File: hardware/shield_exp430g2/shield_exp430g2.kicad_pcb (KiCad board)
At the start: 2 copper layers, 58.7 x 51.2 mm, 45 parts, among them J1 Digital, J10 Conn_01x02_Male, J11 Conn_01x02_Male, J12 Conn_01x02_Male, J13 Conn_01x02_Male, J14 Conn_01x04_Male, J15 Conn_01x02_Male, J16 Conn_01x02_Male, J17 Conn_01x02_Male, J18 Conn_01x02_Male, J19 Conn_01x02_Male, J2 Digital, J20 Conn_01x02_Male, J21 Conn_01x02_Male, J22 Conn_01x02_Male, J23 Conn_01x02_Male, J24 Conn_01x02_Male, J3 Conn_01x02_Male, J4 Conn_01x02_Male, J5 Conn_01x02_Male, J6 Conn_01x02_Male, J7 Conn_01x02_Male, J8 Conn_01x02_Male, J9 Conn_02x13_Odd_Even, U1 NCP1117-3.3_SOT223

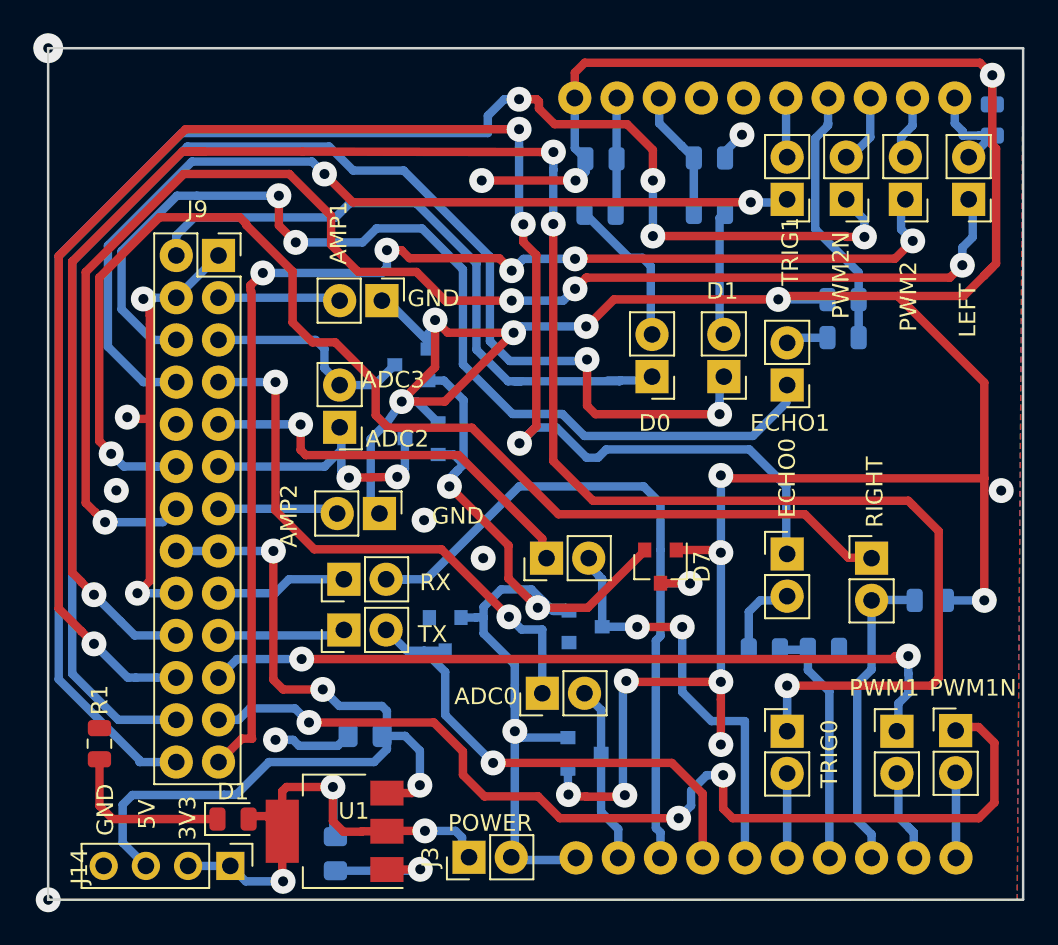
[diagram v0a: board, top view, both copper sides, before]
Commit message: Added diode
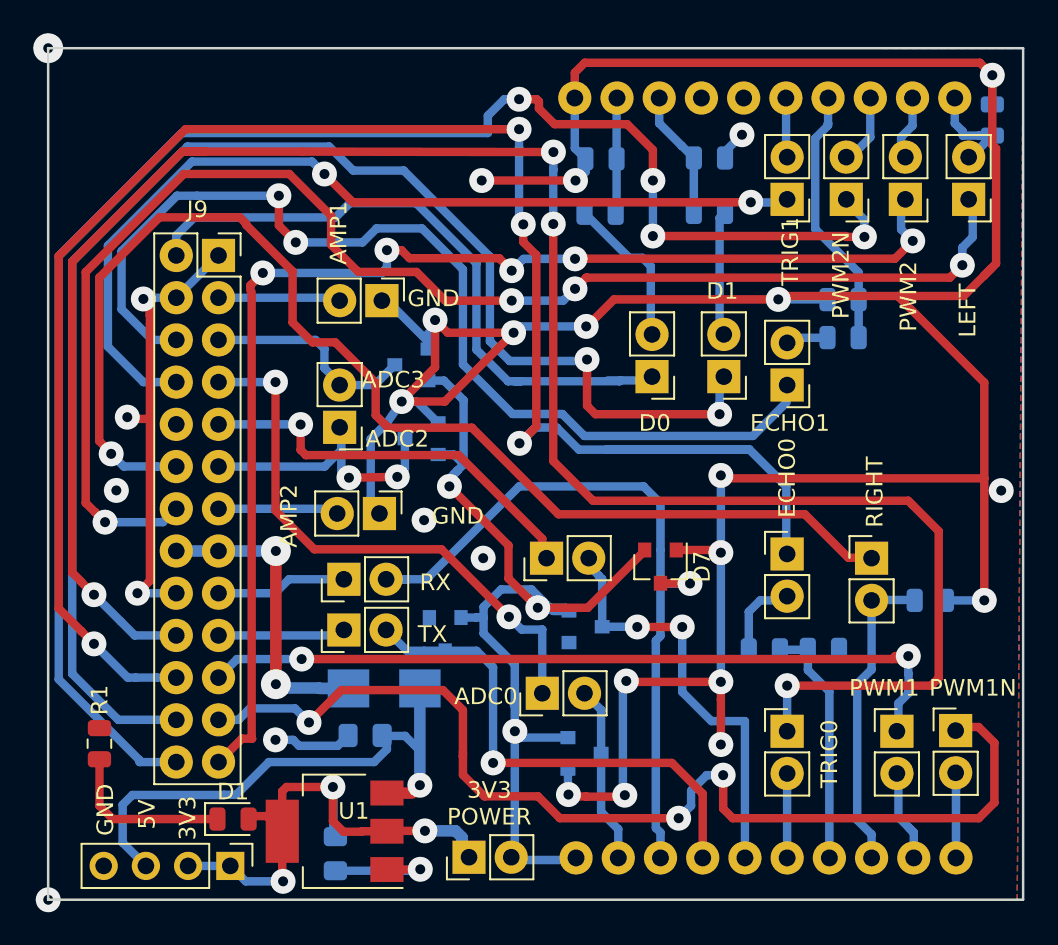
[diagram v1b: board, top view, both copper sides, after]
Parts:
- added D8: D_Schottky, Diode_SMD:D_SMB, B.Cu at (129.9, 113.6)
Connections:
- J9 pad 15: +5V -> +5VP
- J9 pad 16: +5V -> +5VP
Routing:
- net +5VP: track 0.00 -> 18.8 mm, vias 0 -> 2
- net +5V: track 51.6 -> 34.8 mm, vias 3 -> 1
- net Echo0: track 103.3 -> 111.5 mm
- net PWM1N: track 61.1 -> 64.5 mm
- net Net-(C2-Pad1): track 32.9 -> 34.3 mm
- net P1.2: track 29.8 -> 30.5 mm
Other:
- board text added: "3V3 POWER"
- board text removed: "POWER"
